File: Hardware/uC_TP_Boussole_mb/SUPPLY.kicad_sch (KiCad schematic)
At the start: 11 parts, among them J401 Conn_01x02, U401 173010542, U402 AMS1117-3.3

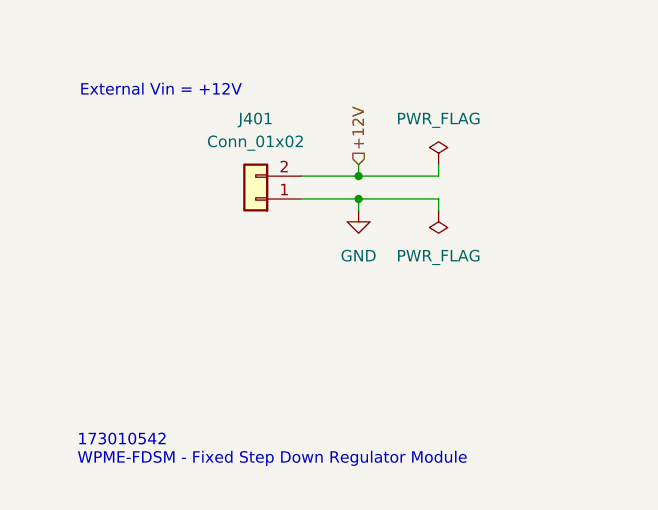
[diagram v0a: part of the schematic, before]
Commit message: ddd
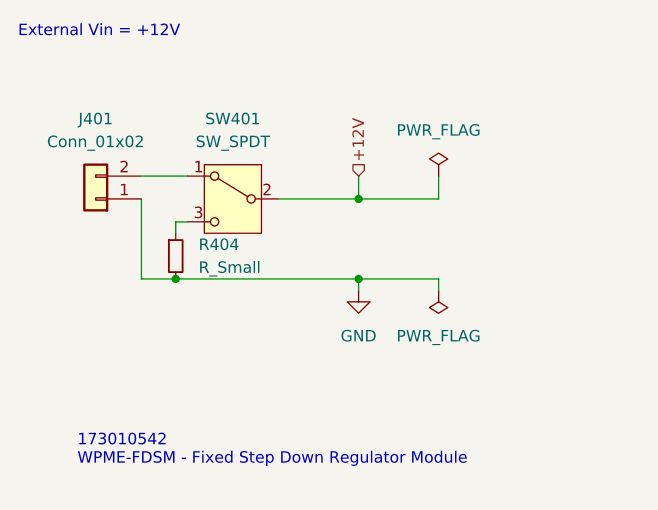
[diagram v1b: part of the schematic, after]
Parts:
- added R404: R_Small, symbol Device:R_Small
- added SW401: SW_SPDT, symbol Switch:SW_SPDT
- U401: footprint (none) -> libs:173010xxx
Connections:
- net +12V: now also SW401.2 (B); no longer J401.2 (Pin_2)
- net GND: now also R404.2
- new net: J401.2 (Pin_2), SW401.1 (A)
- new net: R404.1, SW401.3 (C)
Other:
- moved on the sheet: J401
